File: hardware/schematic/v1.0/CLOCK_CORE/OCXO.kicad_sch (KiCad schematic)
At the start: 13 parts, among them J12 Conn_Coaxial, U6 OCXO-10M

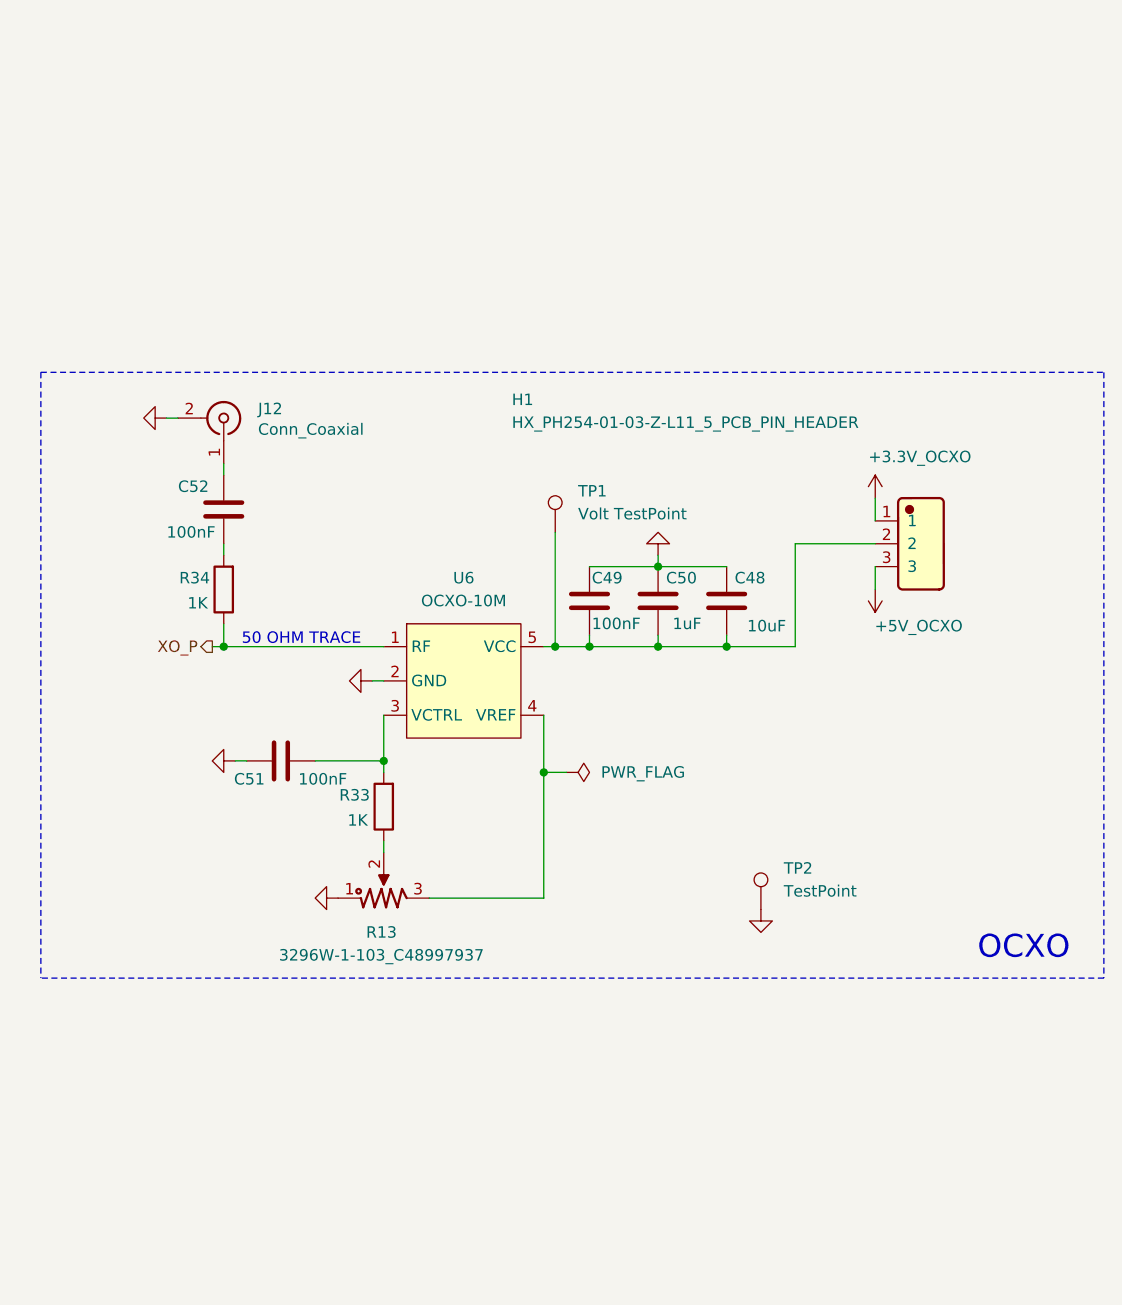
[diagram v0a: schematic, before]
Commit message: sch update
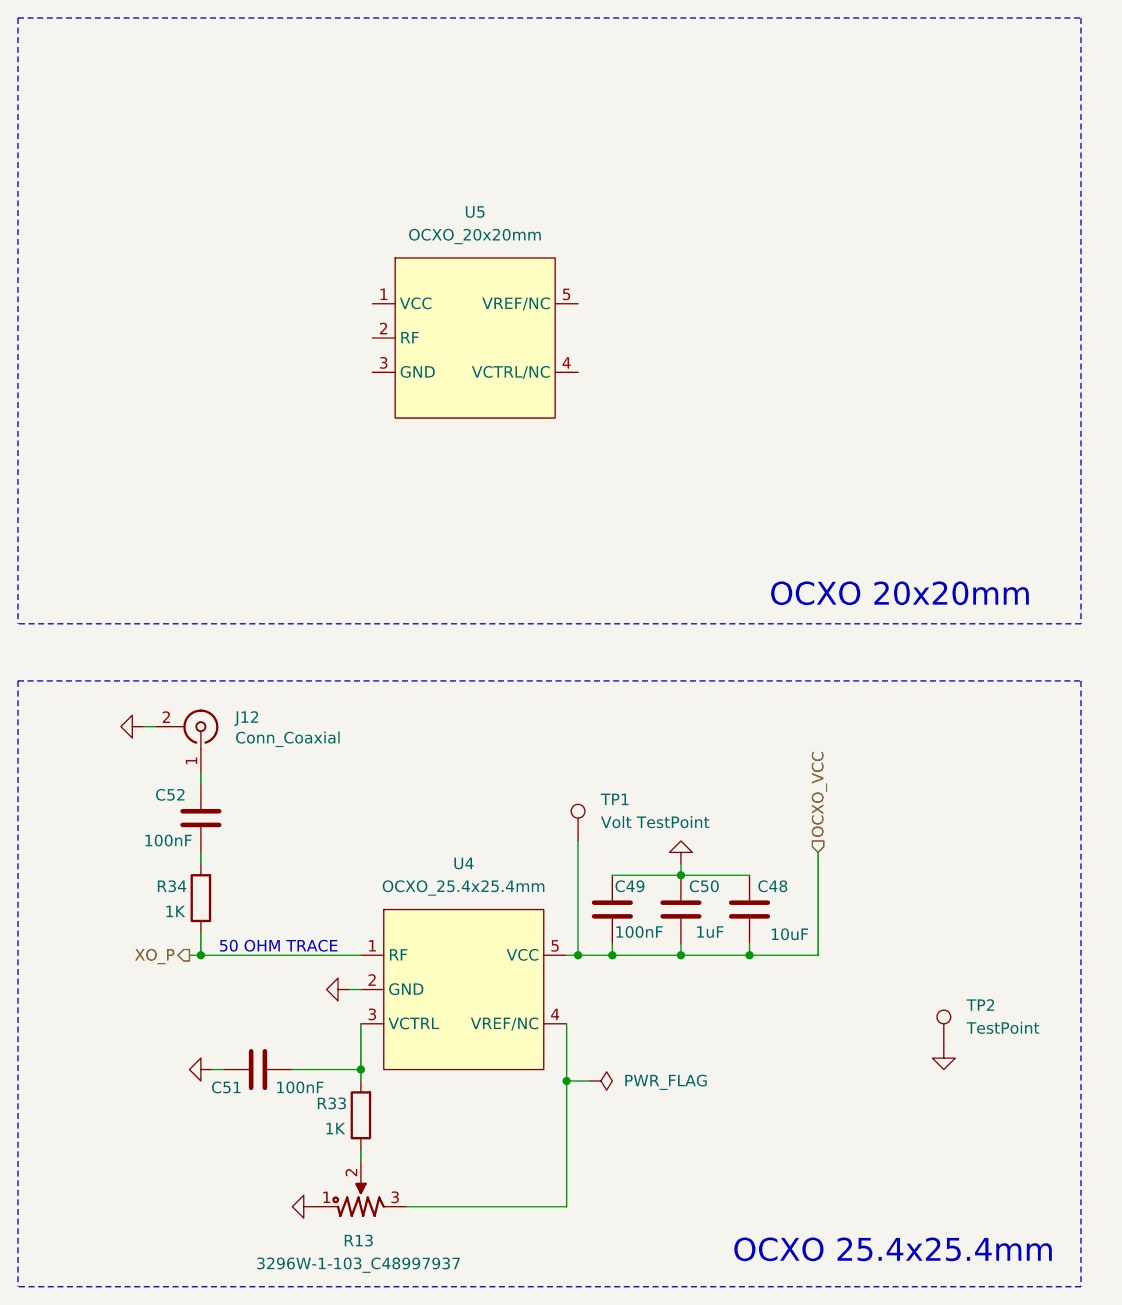
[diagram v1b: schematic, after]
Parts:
- removed H1: HX_PH254-01-03-Z-L11_5_PCB_PIN_HEADER, JLCImport:HX_PH254-01-03-Z-L11_5_PCB_PIN_HEADER, symbol JLCImport:HX_PH254-01-03-Z-L11_5_PCB_PIN_HEADER
- removed U6: OCXO-10M, JLCImport:DOPFITKR2-10M, symbol Counter:OCXO-10M
- added U4: OCXO_25.4x25.4mm, JLCImport:DOPFITKR2-10M, symbol Counter:OCXO_25.4x25.4mm
- added U5: OCXO_20x20mm, JLCImport:OCXO_20x20mm, symbol Counter:OCXO_20x20mm
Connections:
- net GND: now also U4.2 (GND)
- net XO_P: now also U4.1 (RF)
- net at C51.1, R33.2: now also U4.3 (VCTRL)
- net OCXO_VCC: now reaches C48.2, C49.1, C50.2, TP1.1
- net OCXO_VCC: now also U4.5 (VCC)
- net at R13.3: now also U4.4 (VREF/NC)
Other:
- note added: "OCXO 20x20mm"
- note added: "OCXO 25.4x25.4mm"
- note removed: "OCXO"
- moved on the sheet: C48, C49, C50, C51, C52, J12, R13, R33, R34, TP1, TP2
